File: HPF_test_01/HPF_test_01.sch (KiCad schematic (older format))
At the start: 11 parts, among them J1_BNC1 BNC5-J-P-GN-RA-BH2D, J2_BLACK1 Conn_01x01, J3_RED1 Conn_01x01, T1 GT07-110-013, U1 SL1002A600SP

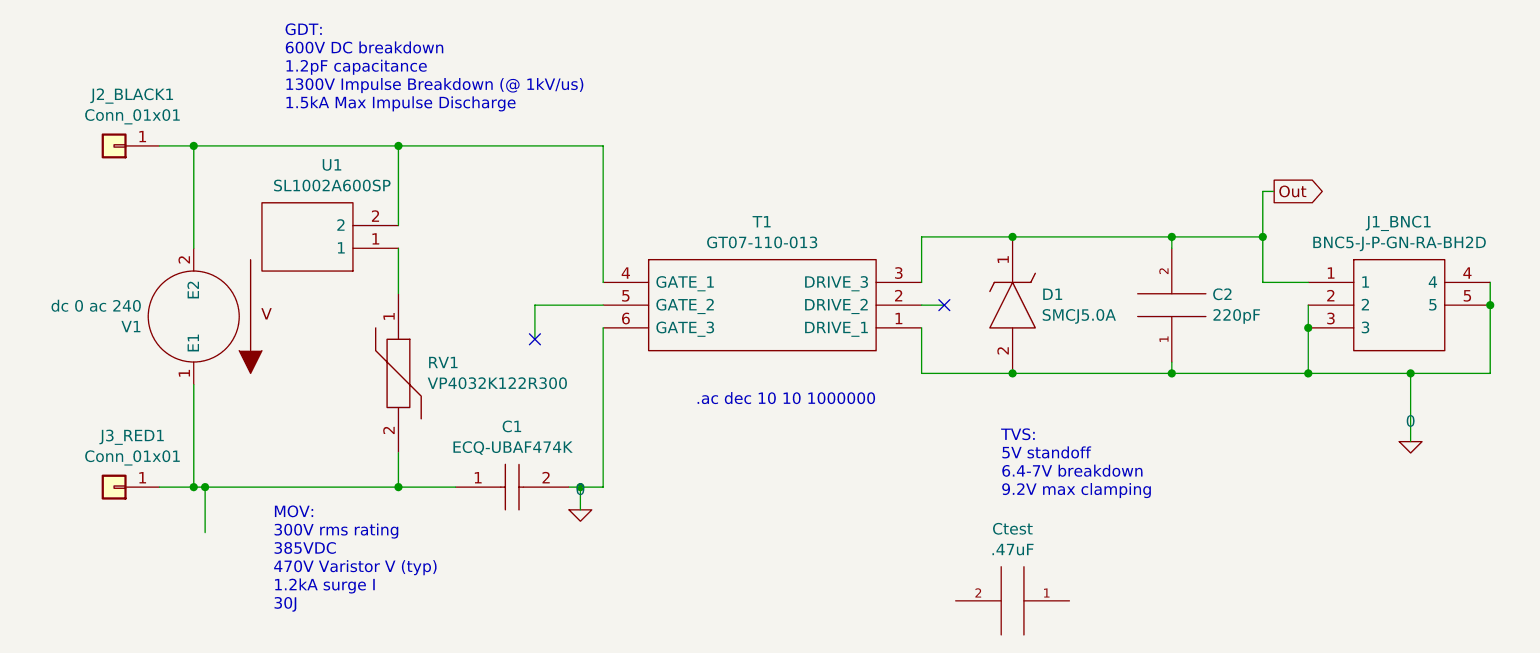
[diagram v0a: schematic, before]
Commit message: Modified 3D render, Added spice outputin test screenshots
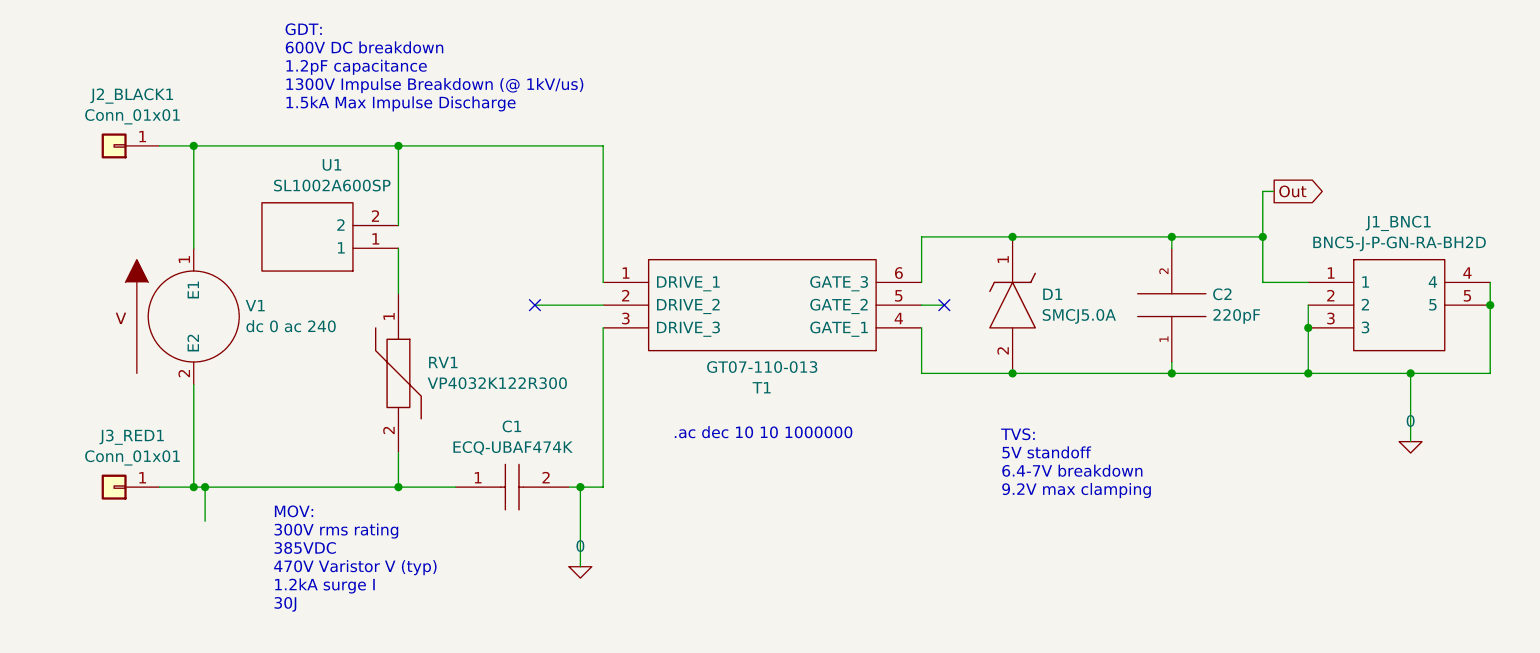
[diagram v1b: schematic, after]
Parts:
- removed Ctest: .47uF, symbol pspice:C
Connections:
- wire segments 42 -> 41
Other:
- moved on the sheet: V1
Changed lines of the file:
@@
 Comment4 ""
 $EndDescr
-Text Notes 6150 4750 2    50   ~ 0
+Text Notes 6050 4900 2    50   ~ 0
 .ac dec 10 10 1000000
 $Comp
@@
 	-1   0    0    1
 $EndComp
-Wire Wire Line
-	4950 3600 4950 4200
 Wire Wire Line
 	4950 5100 4850 5100
@@
 	7450 4000 7850 4000
 Wire Wire Line
-	6350 4400 6350 4600
-Wire Wire Line
 	6350 4600 6750 4600
 Wire Wire Line
@@
 	7450 4550 7450 4600
 Connection ~ 7450 4600
-Wire Wire Line
-	7450 4600 8050 4600
 Wire Wire Line
 	8850 4300 8850 4600
@@
 L GT07-110-013:GT07-110-013 T1
 U 1 1 61D390B4
-P 4950 4200
-F 0 "T1" H 5650 4465 50  0000 C CNN
-F 1 "GT07-110-013" H 5650 4374 50  0000 C CNN
-F 2 "GT07-110-013-Modifed:GT07110013" H 6200 4300 50  0001 L CNN
-F 3 "https://componentsearchengine.com/Datasheets/1/GT07-110-013.pdf" H 6200 4200 50  0001 L CNN
-F 4 "Pulse Transformers" H 6200 4100 50  0001 L CNN "Description"
-F 5 "6.35" H 6200 4000 50  0001 L CNN "Height"
-F 6 "911-GT07-110-013" H 6200 3900 50  0001 L CNN "Mouser Part Number"
-F 7 "https://www.mouser.co.uk/ProductDetail/ICE-Components/GT07-110-013?qs=UkDUCjYnTB00rEvMCOsFKQ%3D%3D" H 6200 3800 50  0001 L CNN "Mouser Price/Stock"
-F 8 "ICE Components" H 6200 3700 50  0001 L CNN "Manufacturer_Name"
-F 9 "GT07-110-013" H 6200 3600 50  0001 L CNN "Manufacturer_Part_Number"
-F 10 "X" H 4950 4200 50  0001 C CNN "Spice_Primitive"
-F 11 "GTRANS" H 4950 4200 50  0001 C CNN "Spice_Model"
-F 12 "Y" H 4950 4200 50  0001 C CNN "Spice_Netlist_Enabled"
-F 13 "/Users/MacMini/Documents/KiCad/HPF/HPF_SPICE/GTRANS_01.lib" H 4950 4200 50  0001 C CNN "Spice_Lib_File"
-	1    4950 4200
-	1    0    0    -1
-$EndComp
-$Comp
-L pspice:0 #GND?
+P 6350 4400
+F 0 "T1" H 7050 4665 50  0000 C CNN
+F 1 "GT07-110-013" H 7050 4574 50  0000 C CNN
+F 2 "GT07-110-013-Modifed:GT07110013" H 7600 4500 50  0001 L CNN
+F 3 "https://componentsearchengine.com/Datasheets/1/GT07-110-013.pdf" H 7600 4400 50  0001 L CNN
+F 4 "Pulse Transformers" H 7600 4300 50  0001 L CNN "Description"
+F 5 "6.35" H 7600 4200 50  0001 L CNN "Height"
+F 6 "911-GT07-110-013" H 7600 4100 50  0001 L CNN "Mouser Part Number"
+F 7 "https://www.mouser.co.uk/ProductDetail/ICE-Components/GT07-110-013?qs=UkDUCjYnTB00rEvMCOsFKQ%3D%3D" H 7600 4000 50  0001 L CNN "Mouser Price/Stock"
+F 8 "ICE Components" H 7600 3900 50  0001 L CNN "Manufacturer_Name"
+F 9 "GT07-110-013" H 7600 3800 50  0001 L CNN "Manufacturer_Part_Number"
+F 10 "X" H 6350 4400 50  0001 C CNN "Spice_Primitive"
+F 11 "GTRANS" H 6350 4400 50  0001 C CNN "Spice_Model"
+F 12 "Y" H 6350 4400 50  0001 C CNN "Spice_Netlist_Enabled"
+F 13 "/Users/MacMini/Documents/KiCad/HPF/HPF_SPICE/GTRANS_01.lib" H 6350 4400 50  0001 C CNN "Spice_Lib_File"
+	1    6350 4400
+	-1   0    0    1
+$EndComp
+$Comp
+L pspice:0 #GND0101
 U 1 1 61D5C253
 P 8500 4900
-F 0 "#GND?" H 8500 4800 50  0001 C CNN
+F 0 "#GND0101" H 8500 4800 50  0001 C CNN
 F 1 "0" H 8500 4989 50  0000 C CNN
 F 2 "" H 8500 4900 50  0001 C CNN
@@
 F 3 "~" H 3150 4350 50  0001 C CNN
 	1    3150 4350
-	-1   0    0    1
-$EndComp
-Wire Wire Line
-	3200 5300 3200 5100
-Connection ~ 3200 5100
-Wire Wire Line
-	3200 5100 4050 5100
+	1    0    0    -1
+$EndComp
 Wire Wire Line
 	3150 4650 3150 5100
 Connection ~ 3150 5100
-Wire Wire Line
-	3150 5100 3200 5100
 Wire Wire Line
 	3150 4050 3150 3600
@@
 Connection ~ 7850 4000
 $Comp
-L pspice:C Ctest
-U 1 1 61D7329D
-P 6750 5600
-F 0 "Ctest" V 6435 5600 50  0000 C CNN
-F 1 ".47uF" V 6526 5600 50  0000 C CNN
-F 2 "" H 6750 5600 50  0001 C CNN
-F 3 "~" H 6750 5600 50  0001 C CNN
-F 4 "C" H 6750 5600 50  0001 C CNN "Spice_Primitive"
-F 5 ".47u" H 6750 5600 50  0001 C CNN "Spice_Model"
-F 6 "N" H 6750 5600 50  0001 C CNN "Spice_Netlist_Enabled"
-	1    6750 5600
-	0    1    1    0
-$EndComp
-$Comp
-L pspice:0 #GND?
+L pspice:0 #GND0102
 U 1 1 61D77CD5
-P 4850 5200
-F 0 "#GND?" H 4850 5100 50  0001 C CNN
-F 1 "0" H 4850 5289 50  0000 C CNN
-F 2 "" H 4850 5200 50  0001 C CNN
-F 3 "~" H 4850 5200 50  0001 C CNN
-	1    4850 5200
+P 4850 5450
+F 0 "#GND0102" H 4850 5350 50  0001 C CNN
+F 1 "0" H 4850 5539 50  0000 C CNN
+F 2 "" H 4850 5450 50  0001 C CNN
+F 3 "~" H 4850 5450 50  0001 C CNN
+	1    4850 5450
 	1    0    0    -1
 $EndComp
@@
 	4950 4300 4650 4300
 Wire Wire Line
-	4650 4300 4650 4450
-Wire Wire Line
 	6450 4300 6350 4300
-Wire Wire Line
-	4850 5200 4850 5100
 Connection ~ 4850 5100
 Wire Wire Line
 	4850 5100 4800 5100
+Wire Wire Line
+	7450 4600 8050 4600
+Wire Wire Line
+	6350 4400 6350 4600
+Wire Wire Line
+	4950 3600 4950 4200
+Wire Wire Line
+	3150 5100 3200 5100
 NoConn ~ 6450 4300
-NoConn ~ 4650 4450
+NoConn ~ 4650 4300
+Wire Wire Line
+	3200 5250 3200 5100
+Connection ~ 3200 5100
+Wire Wire Line
+	3200 5100 4050 5100
+Wire Wire Line
+	4850 5100 4850 5450
 $EndSCHEMATC
